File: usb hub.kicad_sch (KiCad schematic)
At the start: 22 parts, among them J1 TYPE_C, U1 FE1.1s

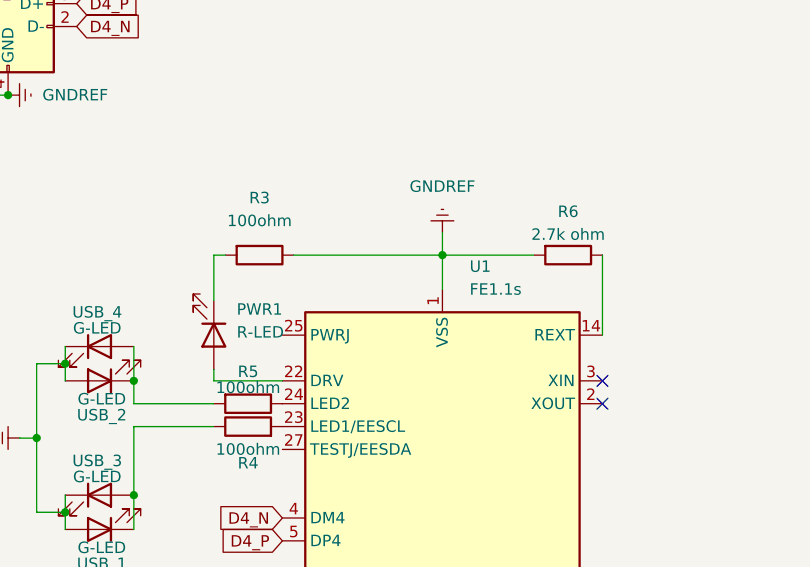
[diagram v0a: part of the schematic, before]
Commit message: bit of routing
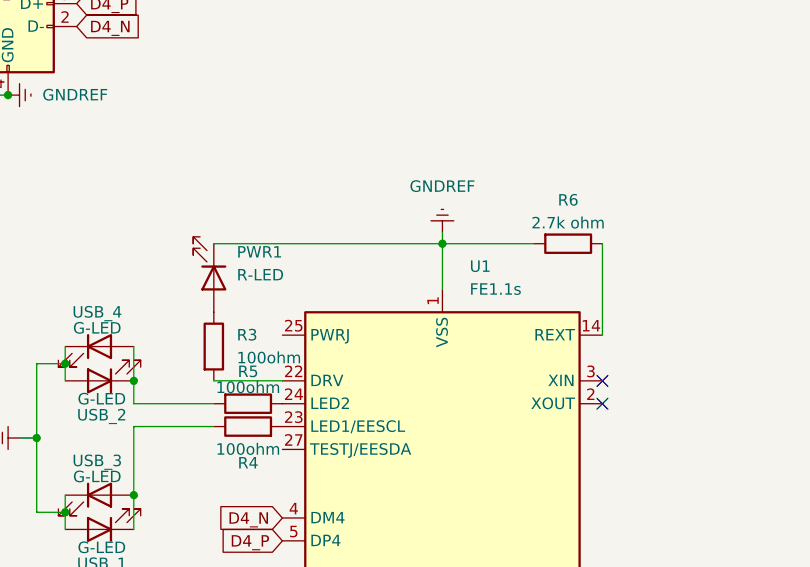
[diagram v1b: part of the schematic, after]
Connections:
- net GND: now also PWR1.1 (K); no longer R3.1
- net at R3.2: now also U1.22 (DRV); no longer PWR1.1 (K)
- net at PWR1.2 (A): now also R3.1; no longer U1.22 (DRV)
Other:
- moved on the sheet: PWR1, R6
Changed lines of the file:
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@@
 	)
 	(junction
-		(at 123.19 100.33)
-		(diameter 0)
-		(color 0 0 0 0)
-	)
-	(junction
 		(at 121.92 160.02)
 		(diameter 0)
@@
 	)
 	(junction
+		(at 123.19 99.06)
+		(diameter 0)
+		(color 0 0 0 0)
+	)
+	(junction
 		(at 88.9 114.3)
 		(diameter 0)
@@
 	(wire
 		(pts
-			(xy 97.79 113.03) (xy 97.79 114.3)
+			(xy 44.45 82.55) (xy 46.99 82.55)
 		)
 		(stroke
@@
 	(wire
 		(pts
-			(xy 44.45 82.55) (xy 46.99 82.55)
+			(xy 140.97 149.86) (xy 142.24 149.86)
 		)
 		(stroke
@@
 	(wire
 		(pts
-			(xy 140.97 149.86) (xy 142.24 149.86)
+			(xy 97.79 99.06) (xy 123.19 99.06)
 		)
 		(stroke
@@
 	(wire
 		(pts
-			(xy 97.79 105.41) (xy 97.79 100.33)
-		)
-		(stroke
-			(width 0)
-			(type default)
-		)
-	)
-	(wire
-		(pts
 			(xy 88.9 127) (xy 88.9 119.38)
 		)
@@
 	(wire
 		(pts
-			(xy 140.97 100.33) (xy 140.97 109.22)
+			(xy 140.97 99.06) (xy 140.97 109.22)
 		)
 		(stroke
@@
 	(wire
 		(pts
-			(xy 78.105 112.395) (xy 81.28 112.395)
+			(xy 123.19 99.06) (xy 123.19 104.14)
 		)
 		(stroke
@@
 	(wire
 		(pts
-			(xy 123.19 97.79) (xy 123.19 100.33)
+			(xy 78.105 112.395) (xy 81.28 112.395)
 		)
 		(stroke
@@
 	(wire
 		(pts
-			(xy 106.68 100.33) (xy 123.19 100.33)
+			(xy 123.19 97.79) (xy 123.19 99.06)
 		)
 		(stroke
@@
 	(wire
 		(pts
-			(xy 133.35 100.33) (xy 123.19 100.33)
+			(xy 133.35 99.06) (xy 123.19 99.06)
 		)
 		(stroke
@@
 	(wire
 		(pts
-			(xy 123.19 100.33) (xy 123.19 104.14)
-		)
-		(stroke
-			(width 0)
-			(type default)
-		)
-	)
-	(wire
-		(pts
 			(xy 128.27 162.56) (xy 128.27 160.02)
 		)
@@
 	(wire
 		(pts
-			(xy 97.79 100.33) (xy 99.06 100.33)
-		)
-		(stroke
-			(width 0)
-			(type default)
-		)
-	)
-	(wire
-		(pts
 			(xy 72.39 82.55) (xy 74.93 82.55)
 		)
@@
 	)
 	(symbol
-		(lib_id "Device:R")
-		(at 102.87 100.33 270)
-		(unit 1)
-		(exclude_from_sim no)
-		(in_bom yes)
-		(on_board yes)
-		(dnp no)
-		(fields_autoplaced yes)
-		(property "Reference" "R3"
-			(at 102.87 93.98 90)
-			(effects
-				(font
-					(size 1.27 1.27)
-				)
-			)
-		)
-		(property "Value" "100ohm"
-			(at 102.87 96.52 90)
-			(effects
-				(font
-					(size 1.27 1.27)
-				)
-			)
-		)
-		(property "Footprint" "Resistor_SMD:R_0201_0603Metric"
-			(at 102.87 98.552 90)
-			(effects
-				(font
-					(size 1.27 1.27)
-				)
-				(hide yes)
-			)
-		)
-		(property "Datasheet" "~"
-			(at 102.87 100.33 0)
-			(effects
-				(font
-					(size 1.27 1.27)
-				)
-				(hide yes)
-			)
-		)
-		(property "Description" "Resistor"
-			(at 102.87 100.33 0)
-			(effects
-				(font
-					(size 1.27 1.27)
-				)
-				(hide yes)
-			)
-		)
-		(pin "1"
-		)
-		(pin "2"
-		)
-		(instances
-			(project ""
-				(path "/d6e9f345-7462-4a5d-9cb3-9d4e9bb08c51"
-					(reference "R3")
-					(unit 1)
-				)
-			)
-		)
-	)
-	(symbol
 		(lib_id "Connector:USB_A")
 		(at 46.99 45.72 0)
@@
 	)
 	(symbol
+		(lib_id "Device:R")
+		(at 97.79 110.49 0)
+		(unit 1)
+		(exclude_from_sim no)
+		(in_bom yes)
+		(on_board yes)
+		(dnp no)
+		(fields_autoplaced yes)
+		(property "Reference" "R3"
+			(at 100.33 109.2199 0)
+			(effects
+				(font
+					(size 1.27 1.27)
+				)
+				(justify left)
+			)
+		)
+		(property "Value" "100ohm"
+			(at 100.33 111.7599 0)
+			(effects
+				(font
+					(size 1.27 1.27)
+				)
+				(justify left)
+			)
+		)
+		(property "Footprint" "Resistor_SMD:R_0201_0603Metric"
+			(at 96.012 110.49 90)
+			(effects
+				(font
+					(size 1.27 1.27)
+				)
+				(hide yes)
+			)
+		)
+		(property "Datasheet" "~"
+			(at 97.79 110.49 0)
+			(effects
+				(font
+					(size 1.27 1.27)
+				)
+				(hide yes)
+			)
+		)
+		(property "Description" "Resistor"
+			(at 97.79 110.49 0)
+			(effects
+				(font
+					(size 1.27 1.27)
+				)
+				(hide yes)
+			)
+		)
+		(pin "1"
+		)
+		(pin "2"
+		)
+		(instances
+			(project "usb hub"
+				(path "/d6e9f345-7462-4a5d-9cb3-9d4e9bb08c51"
+					(reference "R3")
+					(unit 1)
+				)
+			)
+		)
+	)
+	(symbol
 		(lib_id "power:GNDREF")
 		(at 82.55 62.23 180)
@@
 	(symbol
 		(lib_id "Device:R")
-		(at 137.16 100.33 270)
+		(at 137.16 99.06 270)
 		(unit 1)
 		(exclude_from_sim no)
@@
 		(dnp no)
 		(property "Reference" "R6"
-			(at 137.16 95.504 90)
+			(at 137.16 94.234 90)
 			(effects
 				(font
@@
 		)
 		(property "Value" "2.7k ohm"
-			(at 137.16 98.044 90)
+			(at 137.16 96.774 90)
 			(effects
 				(font
@@
 		)
 		(property "Footprint" "Resistor_SMD:R_0201_0603Metric"
-			(at 137.16 98.552 90)
+			(at 137.16 97.282 90)
 			(effects
 				(font
@@
 		)
 		(property "Datasheet" "~"
-			(at 137.16 100.33 0)
+			(at 137.16 99.06 0)
 			(effects
 				(font
@@
 		)
 		(property "Description" "Resistor"
-			(at 137.16 100.33 0)
+			(at 137.16 99.06 0)
 			(effects
 				(font
@@
 	(symbol
 		(lib_id "Device:LED")
-		(at 97.79 109.22 270)
+		(at 97.79 102.87 270)
 		(unit 1)
 		(exclude_from_sim no)
@@
 		(on_board yes)
 		(dnp no)
-		(fields_autoplaced yes)
 		(property "Reference" "PWR1"
-			(at 100.33 106.3624 90)
+			(at 100.33 100.0124 90)
 			(effects
 				(font
@@
 		)
 		(property "Value" "R-LED"
-			(at 100.33 108.9024 90)
+			(at 100.33 102.5524 90)
 			(effects
 				(font
@@
 		)
 		(property "Footprint" "Diode_SMD:D_0201_0603Metric"
-			(at 97.79 109.22 0)
+			(at 97.79 102.87 0)
 			(effects
 				(font
@@
 		)
 		(property "Datasheet" "~"
-			(at 97.79 109.22 0)
+			(at 97.79 102.87 0)
 			(effects
 				(font
@@
 		)
 		(property "Description" "Light emitting diode"
-			(at 97.79 109.22 0)
+			(at 97.79 102.87 0)
 			(effects
 				(font
